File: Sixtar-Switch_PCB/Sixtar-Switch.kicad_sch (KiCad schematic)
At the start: 41 parts, among them J1 USB_C_Receptacle

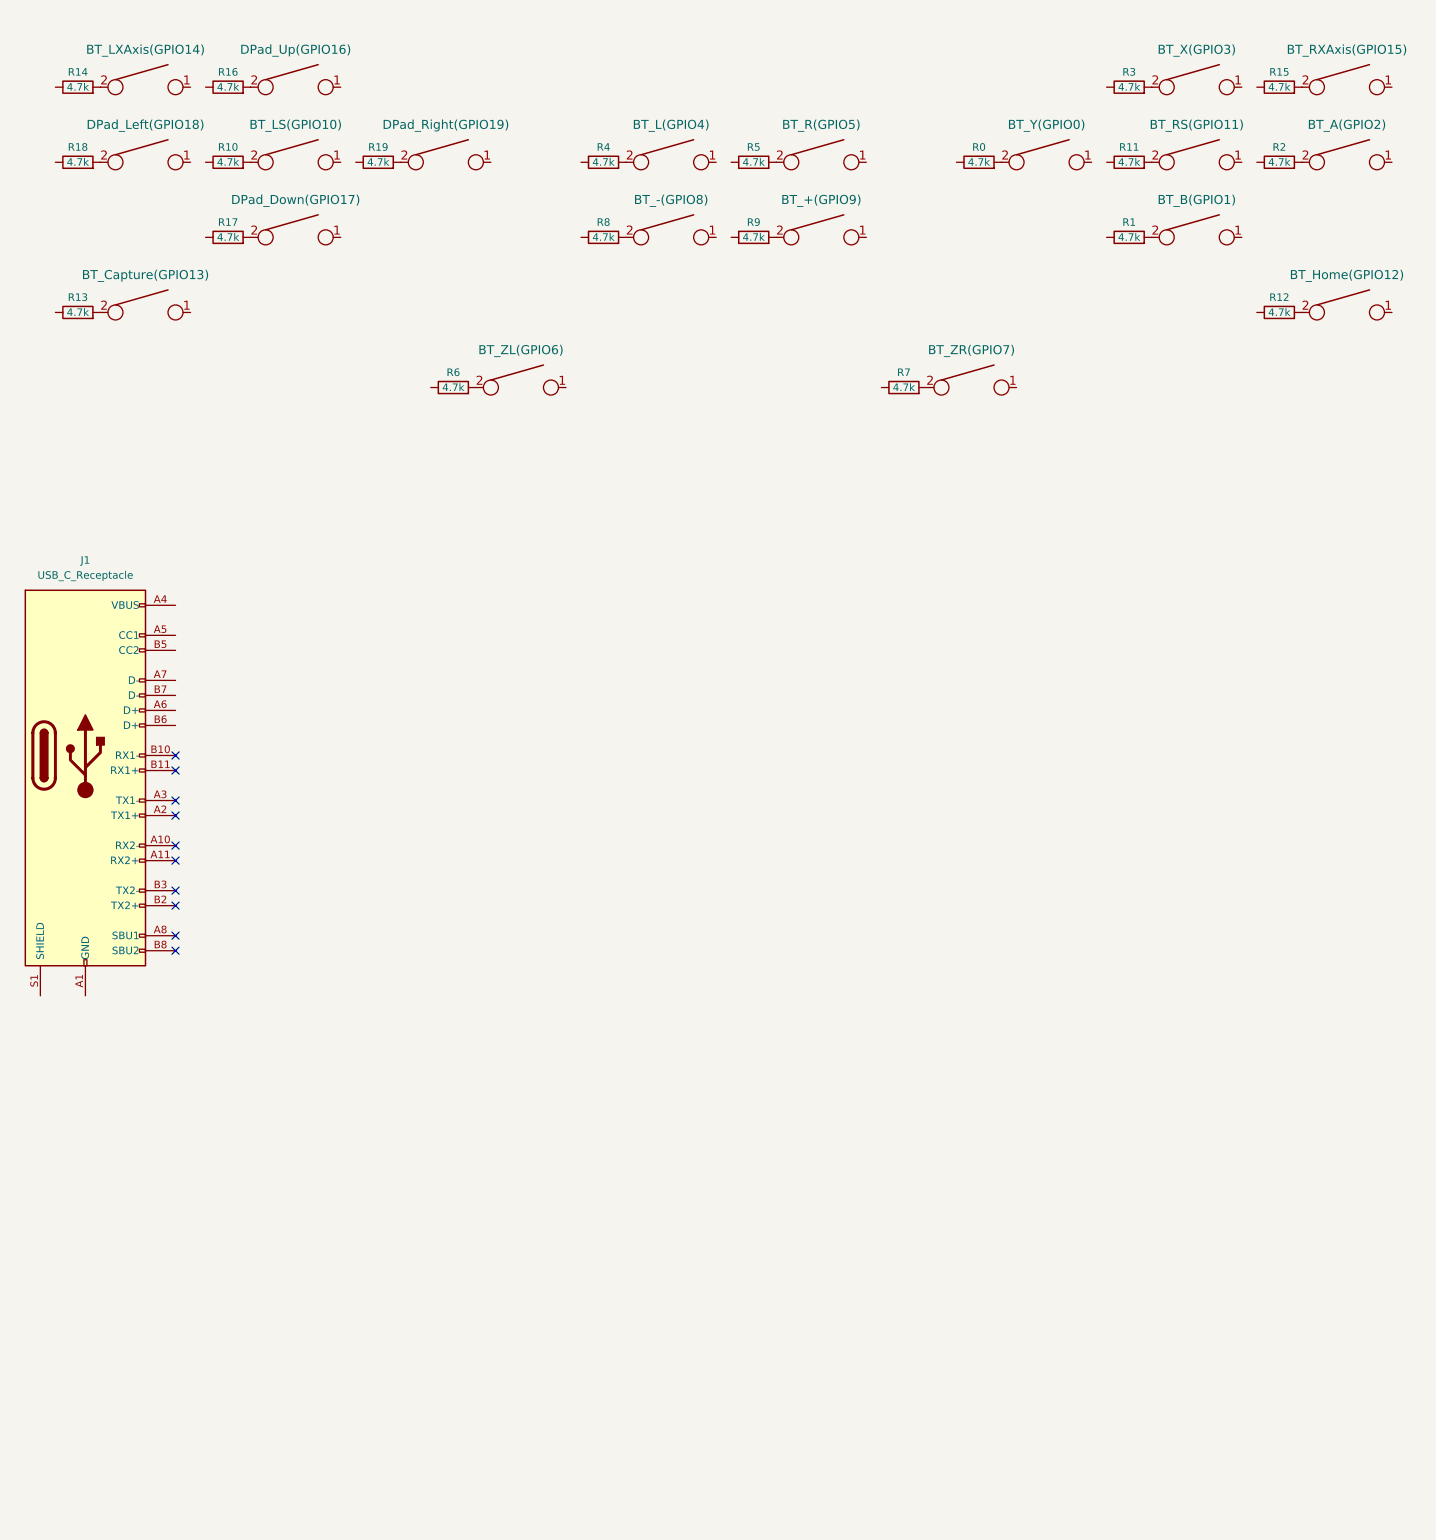
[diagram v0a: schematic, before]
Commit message: kicad 회로 수정
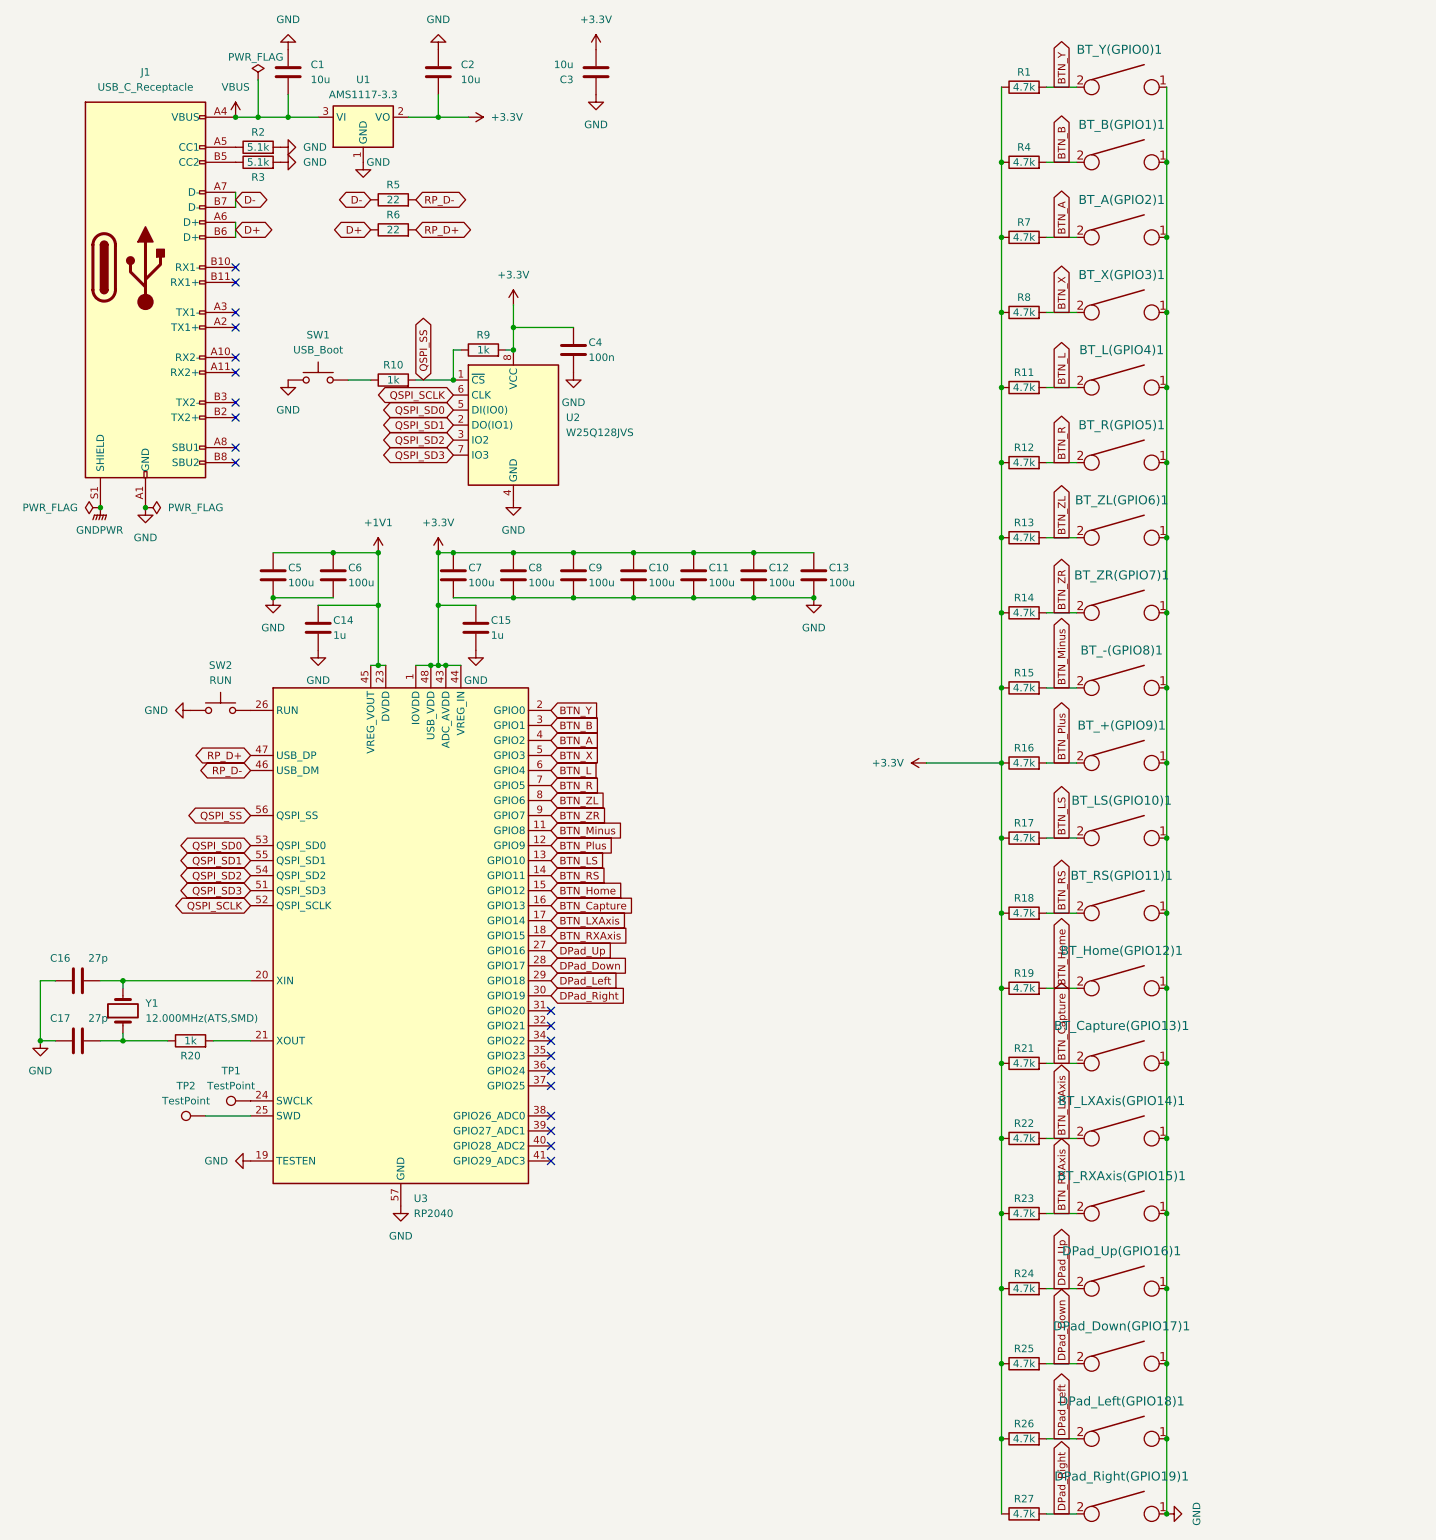
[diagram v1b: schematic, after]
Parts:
- removed R0: 4.7k, symbol Device:R
- added C1, C2, C3: 10u, Capacitor_SMD:C_0805_2012Metric_Pad1.18x1.45mm_HandSolder, symbol Device:C
- added C10, C11, C12, C13, C5, C6, C7, C8, C9: 100u, Capacitor_SMD:C_0805_2012Metric_Pad1.18x1.45mm_HandSolder, symbol Device:C
- added C14, C15: 1u, Capacitor_SMD:C_0805_2012Metric_Pad1.18x1.45mm_HandSolder, symbol Device:C
- added C16, C17: 27p, Capacitor_SMD:C_0805_2012Metric_Pad1.18x1.45mm_HandSolder, symbol Device:C
- added C4: 100n, Capacitor_SMD:C_0805_2012Metric_Pad1.18x1.45mm_HandSolder, symbol Device:C
- added R10, R20, R9: 1k, Resistor_SMD:R_0805_2012Metric_Pad1.20x1.40mm_HandSolder, symbol Device:R
- added R2, R3: 5.1k, Resistor_SMD:R_0805_2012Metric_Pad1.20x1.40mm_HandSolder, symbol Device:R
- added R27: 4.7k, Resistor_SMD:R_0805_2012Metric_Pad1.20x1.40mm_HandSolder, symbol Device:R
- added R5, R6: 22, Resistor_SMD:R_0805_2012Metric_Pad1.20x1.40mm_HandSolder, symbol Device:R
- added SW1: USB_Boot, Connector_PinSocket_2.54mm:PinSocket_1x02_P2.54mm_Vertical, symbol Switch:SW_Push
- added SW2: RUN, Connector_PinSocket_2.54mm:PinSocket_1x02_P2.54mm_Vertical, symbol Switch:SW_Push
- added TP1, TP2: TestPoint, TestPoint:TestPoint_Pad_4.0x4.0mm, symbol Connector:TestPoint
- added U1: AMS1117-3.3, Package_TO_SOT_SMD:SOT-223-3_TabPin2, symbol Regulator_Linear:AMS1117-3.3
- added U2: W25Q128JVS, Package_SO:SOIC-8_5.23x5.23mm_P1.27mm, symbol Memory_Flash:W25Q128JVS
- added U3: RP2040, Package_DFN_QFN:QFN-56-1EP_7x7mm_P0.4mm_EP3.2x3.2mm, symbol MCU_RaspberryPi:RP2040
- added Y1: 12.000MHz(ATS,SMD), Crystal:Crystal_SMD_5032-2Pin_5.0x3.2mm, symbol Device:Crystal
- BT_+(GPIO9)1: renamed from BT_+(GPIO9); footprint (none) -> Button_Switch_Keyboard:SW_Cherry_MX_1.00u_PCB
- BT_-(GPIO8)1: renamed from BT_-(GPIO8); footprint (none) -> Button_Switch_Keyboard:SW_Cherry_MX_1.00u_PCB
- BT_A(GPIO2)1: renamed from BT_A(GPIO2); footprint (none) -> Button_Switch_Keyboard:SW_Cherry_MX_1.00u_PCB
- BT_B(GPIO1)1: renamed from BT_B(GPIO1); footprint (none) -> Button_Switch_Keyboard:SW_Cherry_MX_1.00u_PCB
- BT_Capture(GPIO13)1: renamed from BT_Capture(GPIO13); footprint (none) -> Button_Switch_Keyboard:SW_Cherry_MX_1.00u_PCB
- BT_Home(GPIO12)1: renamed from BT_Home(GPIO12); footprint (none) -> Button_Switch_Keyboard:SW_Cherry_MX_1.00u_PCB
- BT_L(GPIO4)1: renamed from BT_L(GPIO4); footprint (none) -> Button_Switch_Keyboard:SW_Cherry_MX_1.00u_PCB
- BT_LS(GPIO10)1: renamed from BT_LS(GPIO10); footprint (none) -> Button_Switch_Keyboard:SW_Cherry_MX_1.00u_PCB
- BT_LXAxis(GPIO14)1: renamed from BT_LXAxis(GPIO14); footprint (none) -> Button_Switch_Keyboard:SW_Cherry_MX_2.00u_PCB
- BT_R(GPIO5)1: renamed from BT_R(GPIO5); footprint (none) -> Button_Switch_Keyboard:SW_Cherry_MX_1.00u_PCB
- BT_RS(GPIO11)1: renamed from BT_RS(GPIO11); footprint (none) -> Button_Switch_Keyboard:SW_Cherry_MX_1.00u_PCB
- BT_RXAxis(GPIO15)1: renamed from BT_RXAxis(GPIO15); footprint (none) -> Button_Switch_Keyboard:SW_Cherry_MX_2.00u_PCB
- BT_X(GPIO3)1: renamed from BT_X(GPIO3); footprint (none) -> Button_Switch_Keyboard:SW_Cherry_MX_1.00u_PCB
- BT_Y(GPIO0)1: renamed from BT_Y(GPIO0); footprint (none) -> Button_Switch_Keyboard:SW_Cherry_MX_1.00u_PCB
- BT_ZL(GPIO6)1: renamed from BT_ZL(GPIO6); footprint (none) -> Button_Switch_Keyboard:SW_Cherry_MX_2.00u_PCB
- BT_ZR(GPIO7)1: renamed from BT_ZR(GPIO7); footprint (none) -> Button_Switch_Keyboard:SW_Cherry_MX_2.00u_PCB
- DPad_Down(GPIO17)1: renamed from DPad_Down(GPIO17); footprint (none) -> Button_Switch_Keyboard:SW_Cherry_MX_1.00u_PCB
- DPad_Left(GPIO18)1: renamed from DPad_Left(GPIO18); footprint (none) -> Button_Switch_Keyboard:SW_Cherry_MX_1.00u_PCB
- DPad_Right(GPIO19)1: renamed from DPad_Right(GPIO19); footprint (none) -> Button_Switch_Keyboard:SW_Cherry_MX_1.00u_PCB
- DPad_Up(GPIO16)1: renamed from DPad_Up(GPIO16); footprint (none) -> Button_Switch_Keyboard:SW_Cherry_MX_1.00u_PCB
- J1: footprint (none) -> Connector_USB:USB_C_Receptacle_XKB_U262-16XN-4BVC11
- R1: footprint (none) -> Resistor_SMD:R_0805_2012Metric_Pad1.20x1.40mm_HandSolder
- R11: renamed from R5; footprint (none) -> Resistor_SMD:R_0805_2012Metric_Pad1.20x1.40mm_HandSolder
- R12: renamed from R6; footprint (none) -> Resistor_SMD:R_0805_2012Metric_Pad1.20x1.40mm_HandSolder
- R13: renamed from R7; footprint (none) -> Resistor_SMD:R_0805_2012Metric_Pad1.20x1.40mm_HandSolder
- R14: renamed from R8; footprint (none) -> Resistor_SMD:R_0805_2012Metric_Pad1.20x1.40mm_HandSolder
- R15: renamed from R9; footprint (none) -> Resistor_SMD:R_0805_2012Metric_Pad1.20x1.40mm_HandSolder
- R16: renamed from R10; footprint (none) -> Resistor_SMD:R_0805_2012Metric_Pad1.20x1.40mm_HandSolder
- R17: renamed from R11; footprint (none) -> Resistor_SMD:R_0805_2012Metric_Pad1.20x1.40mm_HandSolder
- R18: renamed from R12; footprint (none) -> Resistor_SMD:R_0805_2012Metric_Pad1.20x1.40mm_HandSolder
- R19: renamed from R13; footprint (none) -> Resistor_SMD:R_0805_2012Metric_Pad1.20x1.40mm_HandSolder
- R21: renamed from R14; footprint (none) -> Resistor_SMD:R_0805_2012Metric_Pad1.20x1.40mm_HandSolder
- R22: renamed from R15; footprint (none) -> Resistor_SMD:R_0805_2012Metric_Pad1.20x1.40mm_HandSolder
- R23: renamed from R16; footprint (none) -> Resistor_SMD:R_0805_2012Metric_Pad1.20x1.40mm_HandSolder
- R24: renamed from R17; footprint (none) -> Resistor_SMD:R_0805_2012Metric_Pad1.20x1.40mm_HandSolder
- R25: renamed from R18; footprint (none) -> Resistor_SMD:R_0805_2012Metric_Pad1.20x1.40mm_HandSolder
- R26: renamed from R19; footprint (none) -> Resistor_SMD:R_0805_2012Metric_Pad1.20x1.40mm_HandSolder
- R4: renamed from R2; footprint (none) -> Resistor_SMD:R_0805_2012Metric_Pad1.20x1.40mm_HandSolder
- R7: renamed from R3; footprint (none) -> Resistor_SMD:R_0805_2012Metric_Pad1.20x1.40mm_HandSolder
- R8: renamed from R4; footprint (none) -> Resistor_SMD:R_0805_2012Metric_Pad1.20x1.40mm_HandSolder
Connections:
- net GND: now reaches BT_ZR(GPIO7)1.1
- net GND: now also BT_+(GPIO9)1.1, BT_-(GPIO8)1.1, BT_A(GPIO2)1.1, BT_B(GPIO1)1.1, BT_Capture(GPIO13)1.1, BT_Home(GPIO12)1.1, BT_L(GPIO4)1.1, BT_LS(GPIO10)1.1, BT_LXAxis(GPIO14)1.1, BT_R(GPIO5)1.1, BT_RS(GPIO11)1.1, BT_RXAxis(GPIO15)1.1, BT_X(GPIO3)1.1, BT_Y(GPIO0)1.1, BT_ZL(GPIO6)1.1, DPad_Down(GPIO17)1.1, DPad_Left(GPIO18)1.1, DPad_Right(GPIO19)1.1, DPad_Up(GPIO16)1.1, J1.A1 (GND), J1.A12 (GND), J1.B1 (GND), J1.B12 (GND), C1.1, C10.2, C11.2, C12.2, C13.2, C14.2, C15.2, C16.1, C17.1, C2.1, C3.1, C4.2, C5.2, C6.2, C7.2, C8.2, C9.2, R2.2, R3.2, SW1.1, SW2.1, U1.1 (GND), U2.4 (GND), U3.19 (TESTEN), U3.57 (GND)
- net BTN_ZL: now reaches R13.2
- net BTN_ZL: now also BT_ZL(GPIO6)1.2, U3.8 (GPIO6); no longer BT_ZR(GPIO7)1.2
- net +3.3V: now reaches R11.1
- net +3.3V: now also R1.1, R12.1, R13.1, R14.1, R15.1, R16.1, R17.1, R18.1, R19.1, R21.1, R22.1, R23.1, R24.1, R25.1, R26.1, R4.1, R7.1, R8.1, C10.1, C11.1, C12.1, C13.1, C15.1, C2.2, C3.2, C4.1, C7.1, C8.1, C9.1, R27.1, R9.2, U1.2 (VO), U2.8 (VCC), U3.1 (IOVDD), U3.10 (IOVDD), U3.22 (IOVDD), U3.33 (IOVDD), U3.42 (IOVDD), U3.43 (ADC_AVDD), U3.44 (VREG_IN), U3.48 (USB_VDD), U3.49 (IOVDD)
- net BTN_L: now reaches R11.2
- net BTN_L: now also BT_L(GPIO4)1.2, U3.6 (GPIO4); no longer BT_R(GPIO5)1.2
- net BTN_RXAxis: now reaches R23.2
- net BTN_RXAxis: now also BT_RXAxis(GPIO15)1.2, U3.18 (GPIO15); no longer DPad_Up(GPIO16)1.2
- net BTN_Capture: now reaches BT_Capture(GPIO13)1.2
- net BTN_Capture: now also R21.2, U3.16 (GPIO13); no longer R19.2
- net DPad_Down: now reaches DPad_Down(GPIO17)1.2
- net DPad_Down: now also R25.2, U3.28 (GPIO17); no longer R24.2
- net BTN_LS: now reaches BT_LS(GPIO10)1.2
- net BTN_LS: now also R17.2, U3.13 (GPIO10); no longer R16.2
- net BTN_B: now reaches BT_B(GPIO1)1.2
- net BTN_B: now also R4.2, U3.3 (GPIO1); no longer R1.2
- net BTN_Home: now reaches BT_Home(GPIO12)1.2
- net BTN_Home: now also R19.2, U3.15 (GPIO12); no longer R18.2
- net BTN_RS: now reaches BT_RS(GPIO11)1.2
- net BTN_RS: now also R18.2, U3.14 (GPIO11); no longer R17.2
- net DPad_Left: now reaches DPad_Left(GPIO18)1.2
- net DPad_Left: now also R26.2, U3.29 (GPIO18); no longer R25.2
- net BTN_Y: now reaches BT_Y(GPIO0)1.2
- net BTN_Y: now also R1.2, U3.2 (GPIO0)
- net BTN_LXAxis: now reaches BT_LXAxis(GPIO14)1.2
- net BTN_LXAxis: now also R22.2, U3.17 (GPIO14); no longer R21.2
- net BTN_Minus: now reaches R15.2
- net BTN_Minus: now also BT_-(GPIO8)1.2, U3.11 (GPIO8); no longer BT_+(GPIO9)1.2
- net BTN_R: now reaches R12.2
- net BTN_R: now also BT_R(GPIO5)1.2, U3.7 (GPIO5); no longer BT_ZL(GPIO6)1.2
- net VBUS: now reaches J1.A4 (VBUS), J1.A9 (VBUS), J1.B4 (VBUS), J1.B9 (VBUS)
- net VBUS: now also C1.2, U1.3 (VI)
- net at J1.A5 (CC1): now also R2.1
- net D+: now reaches J1.A6 (D+)
- net D+: now also J1.B6 (D+), R6.1
- net D-: now reaches J1.A7 (D-)
- net D-: now also J1.B7 (D-), R5.1
- net at J1.B5 (CC2): now also R3.1
- net GNDPWR: now reaches J1.S1 (SHIELD)
- net BTN_X: now reaches R8.2
- net BTN_X: now also BT_X(GPIO3)1.2, U3.5 (GPIO3); no longer BT_L(GPIO4)1.2
- net BTN_A: now reaches BT_A(GPIO2)1.2
- net BTN_A: now also R7.2, U3.4 (GPIO2); no longer R4.2
- net BTN_ZR: now reaches R14.2
- net BTN_ZR: now also BT_ZR(GPIO7)1.2, U3.9 (GPIO7); no longer BT_-(GPIO8)1.2
- net DPad_Right: now reaches DPad_Right(GPIO19)1.2
- net DPad_Right: now also R27.2, U3.30 (GPIO19); no longer R26.2
- new net: C17.2, R20.1, Y1.1
- new net: C16.2, U3.20 (XIN), Y1.2
- new net: R20.2, U3.21 (XOUT)
- new net: TP1.1, U3.24 (SWCLK)
- new net: TP2.1, U3.25 (SWD)
- new net: SW2.2, U3.26 (RUN)
- new net: R10.1, SW1.2
- new net +1V1: C14.1, C5.1, C6.1, U3.23 (DVDD), U3.45 (VREG_VOUT), U3.50 (DVDD)
- new net BTN_Plus: BT_+(GPIO9)1.2, R16.2, U3.12 (GPIO9)
- new net DPad_Up: DPad_Up(GPIO16)1.2, R24.2, U3.27 (GPIO16)
- new net QSPI_SCLK: U2.6 (CLK), U3.52 (QSPI_SCLK)
- new net QSPI_SD0: U2.5 (DI(IO0)), U3.53 (QSPI_SD0)
- new net QSPI_SD1: U2.2 (DO(IO1)), U3.55 (QSPI_SD1)
- new net QSPI_SD2: U2.3 (IO2), U3.54 (QSPI_SD2)
- new net QSPI_SD3: U2.7 (IO3), U3.51 (QSPI_SD3)
- new net QSPI_SS: R10.2, R9.1, U2.1 (~{CS}), U3.56 (QSPI_SS)
- new net RP_D+: R6.2, U3.47 (USB_DP)
- new net RP_D-: R5.2, U3.46 (USB_DM)
- no-connect marks 10 -> 20
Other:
- moved on the sheet: BT_+(GPIO9)1, BT_-(GPIO8)1, BT_A(GPIO2)1, BT_B(GPIO1)1, BT_Capture(GPIO13)1, BT_Home(GPIO12)1, BT_L(GPIO4)1, BT_LS(GPIO10)1, BT_LXAxis(GPIO14)1, BT_R(GPIO5)1, BT_RS(GPIO11)1, BT_RXAxis(GPIO15)1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
